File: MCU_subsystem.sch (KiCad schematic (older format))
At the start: 14 parts, among them U601 cc1352p, U602 MX25R8035FZUIL0, Y601 32.768kHz, Y602 48MHz

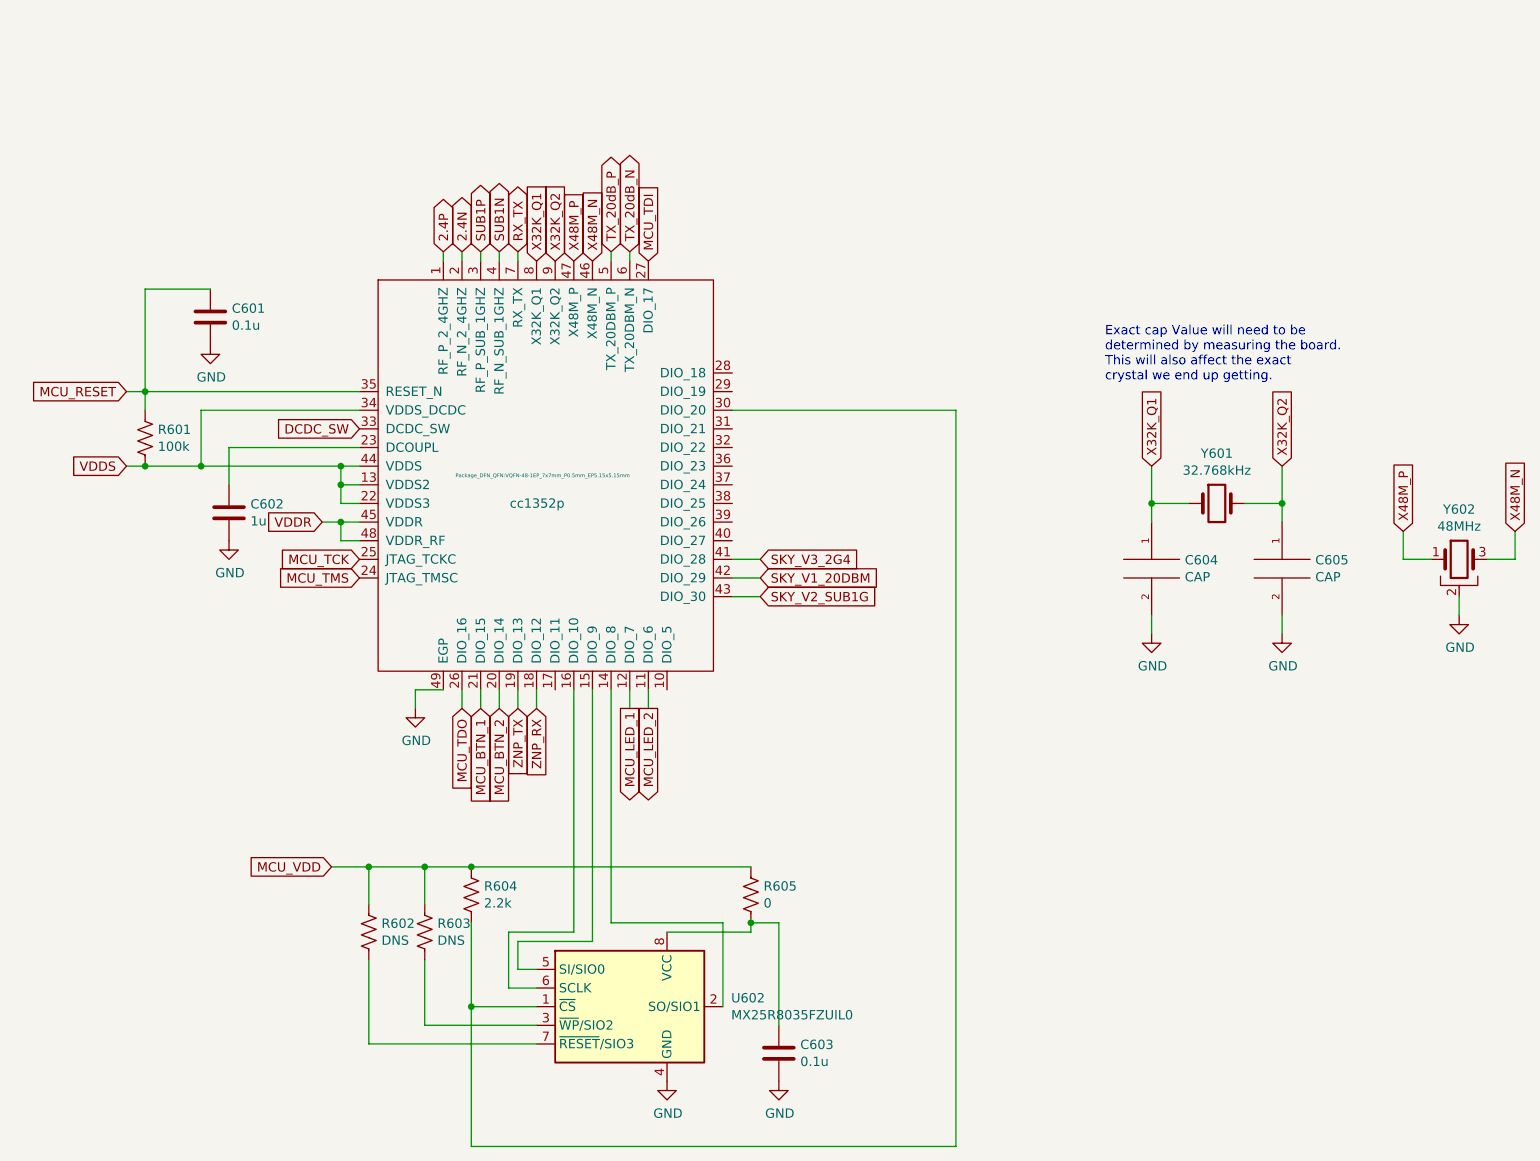
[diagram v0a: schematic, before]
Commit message: final edits before it'll be untouched
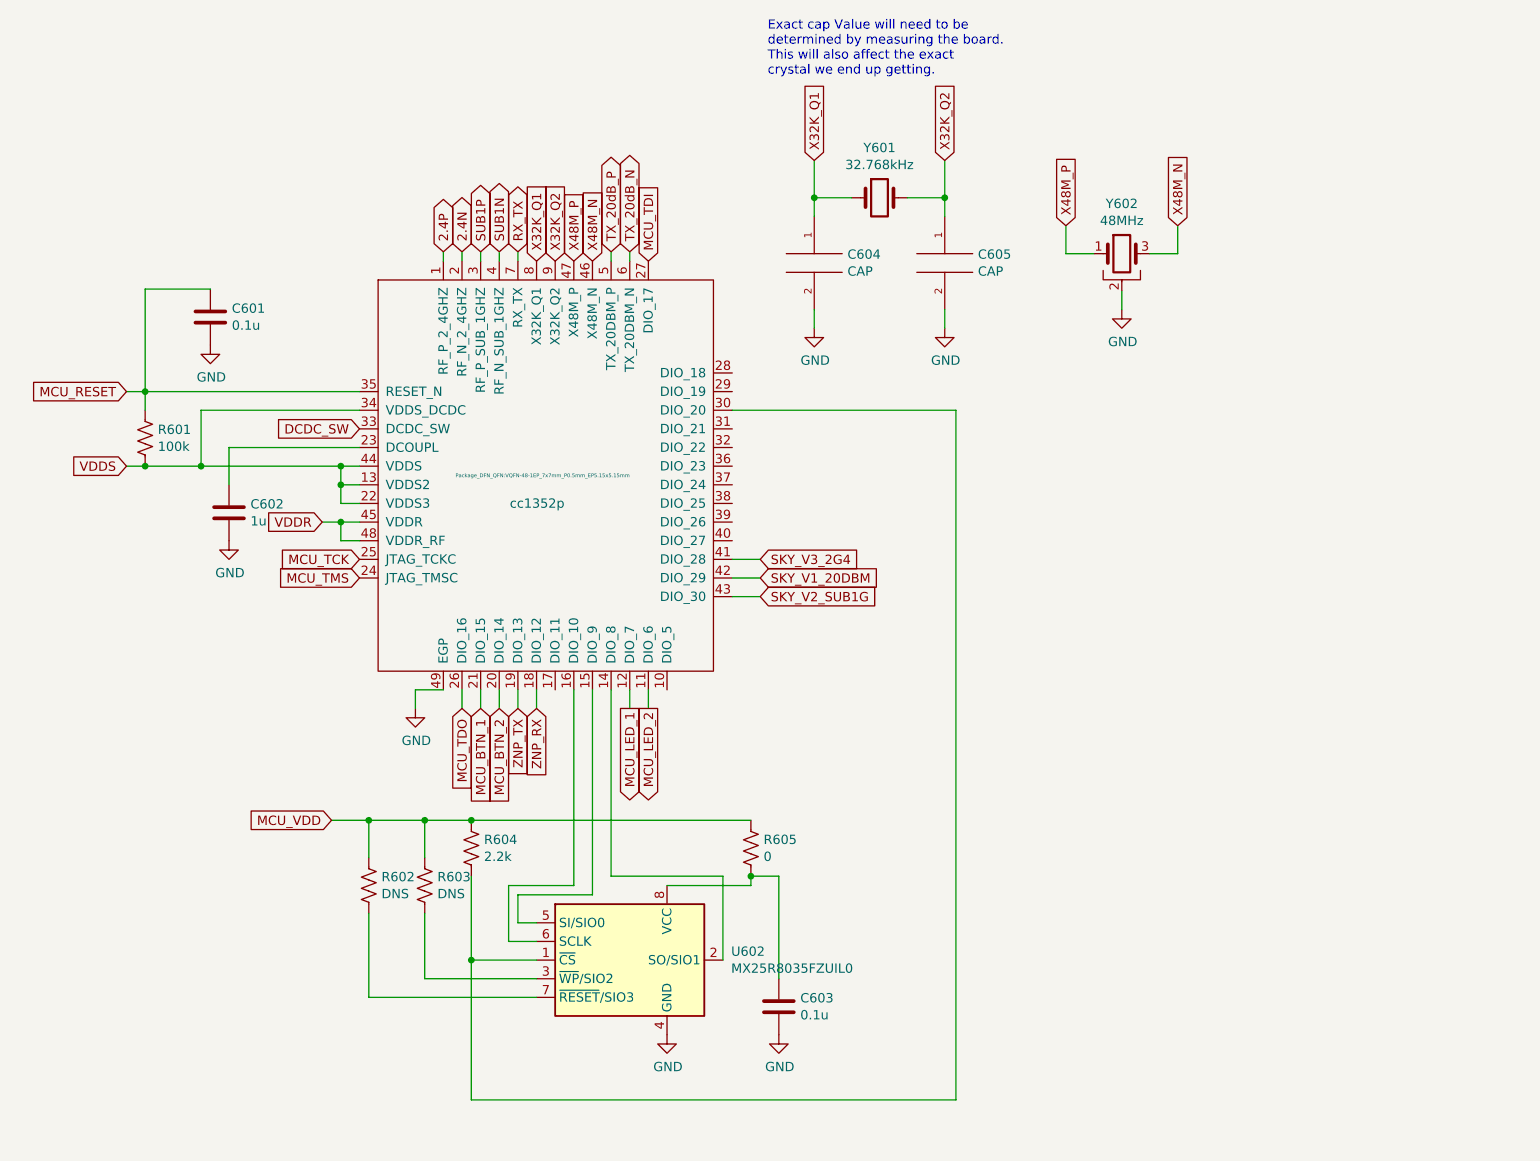
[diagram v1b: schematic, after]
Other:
- moved on the sheet: C603, C604, C605, R602, R603, R604, R605, U602, Y601, Y602
